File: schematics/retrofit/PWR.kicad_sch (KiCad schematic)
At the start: 4 parts, among them J601 24V PWR, U601 7i97-TB4-5V

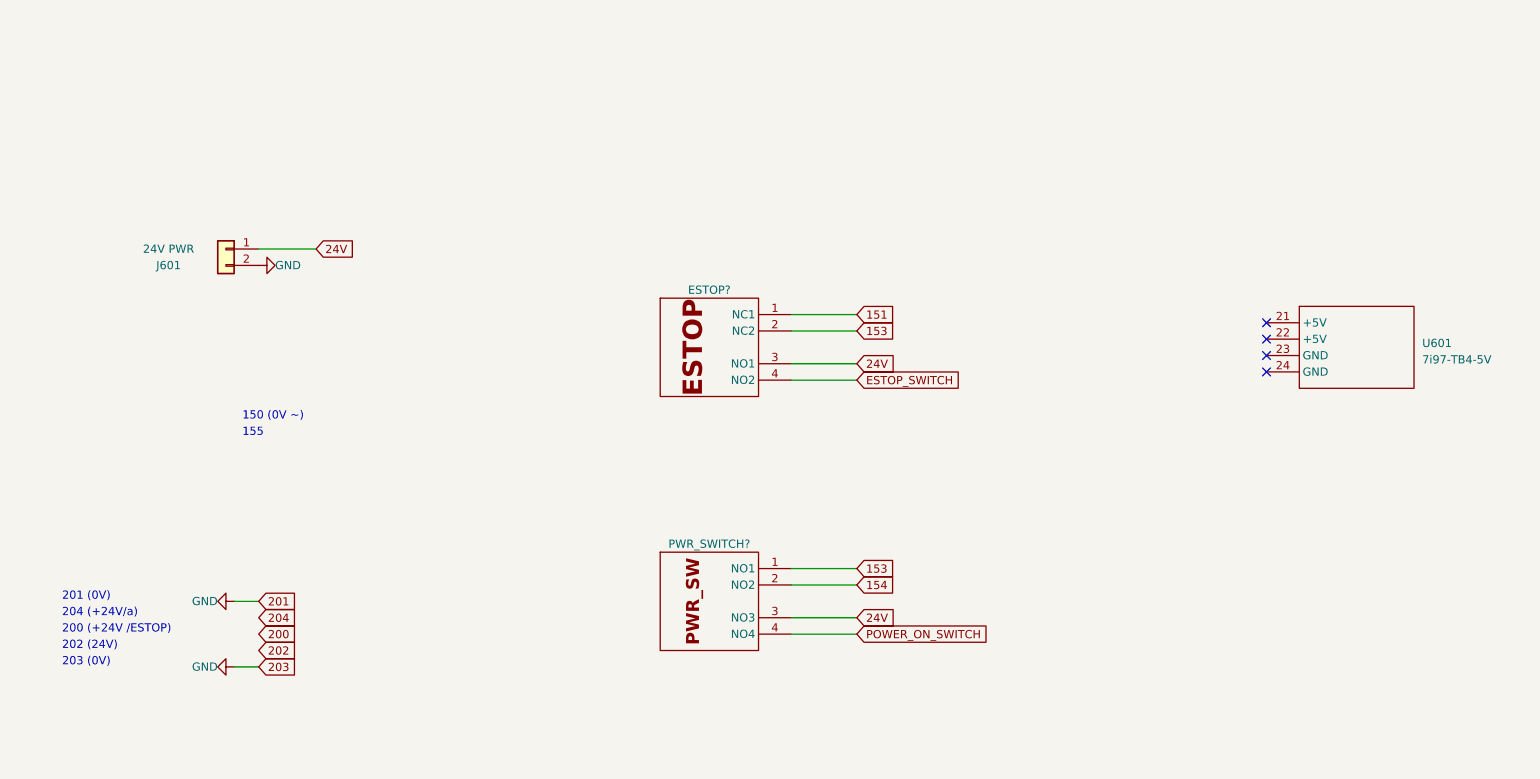
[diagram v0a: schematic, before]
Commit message: schematics
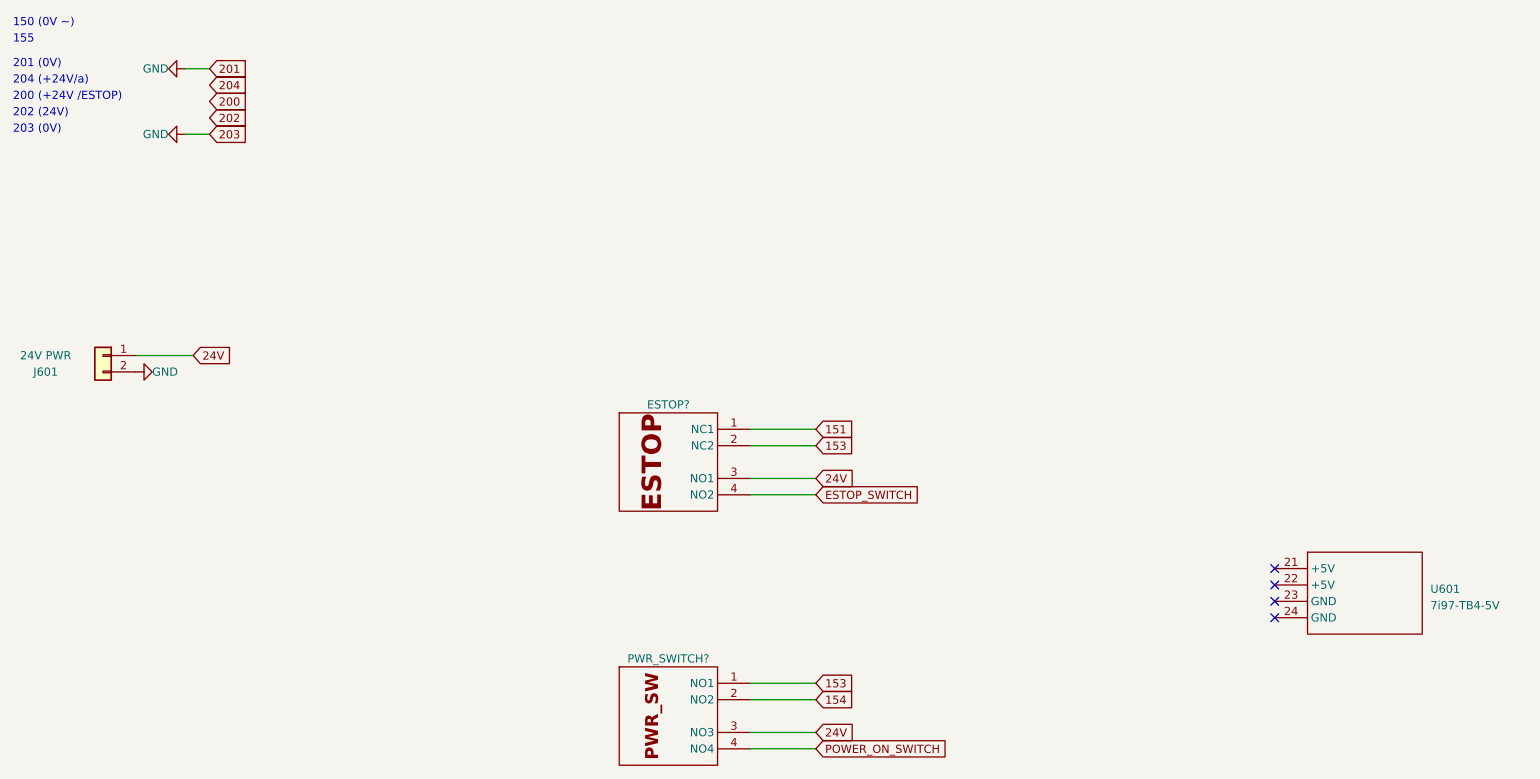
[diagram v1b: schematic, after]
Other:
- moved on the sheet: ESTOP?, J601, PWR_SWITCH?, U601
